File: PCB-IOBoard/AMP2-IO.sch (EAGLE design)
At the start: 85 parts, among them IC1 7404TS, IC2 R-78E6.5-0.5, IC3 REG1117, IC4 REG1117, K2 GN210S03, Q4 24.576, X3 MKDSN1,5/2-5,08

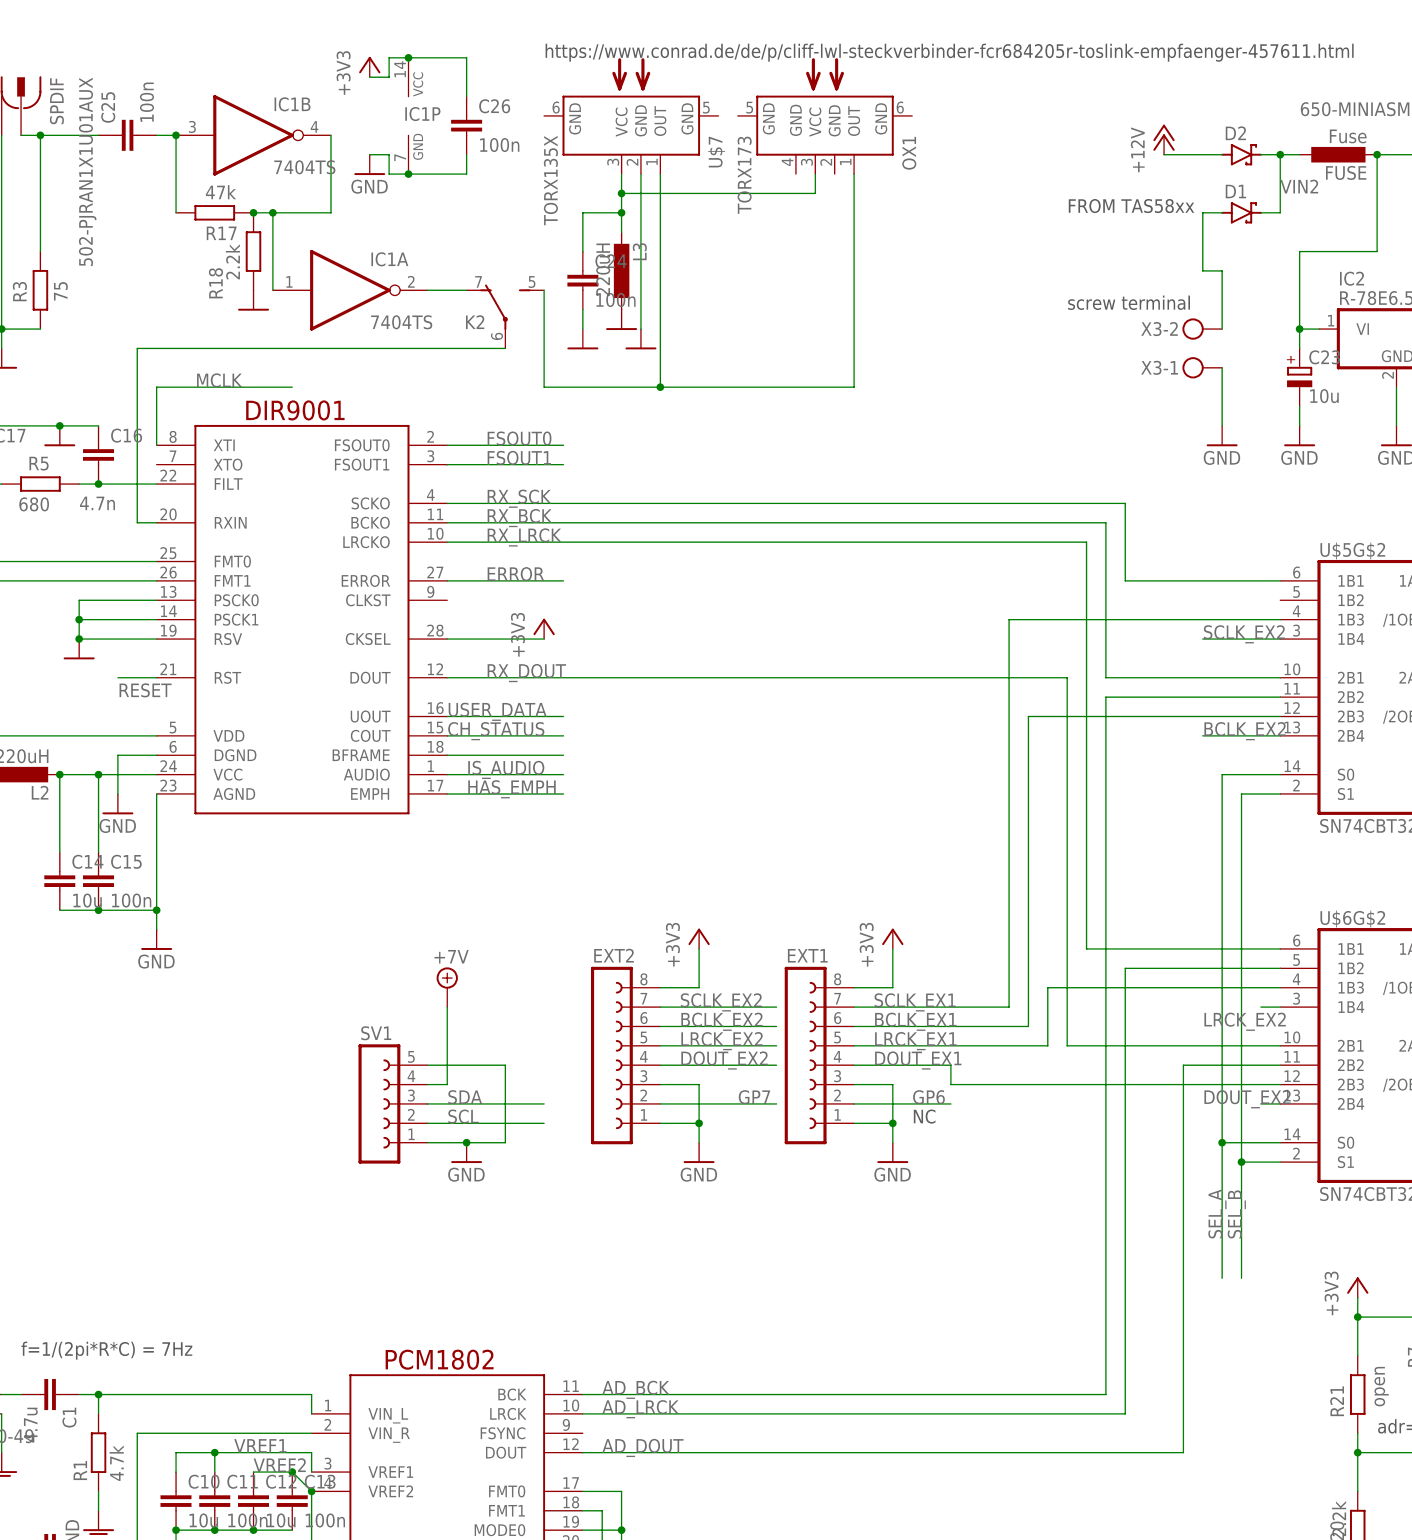
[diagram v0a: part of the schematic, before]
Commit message: Some RC1 bugs fixed.
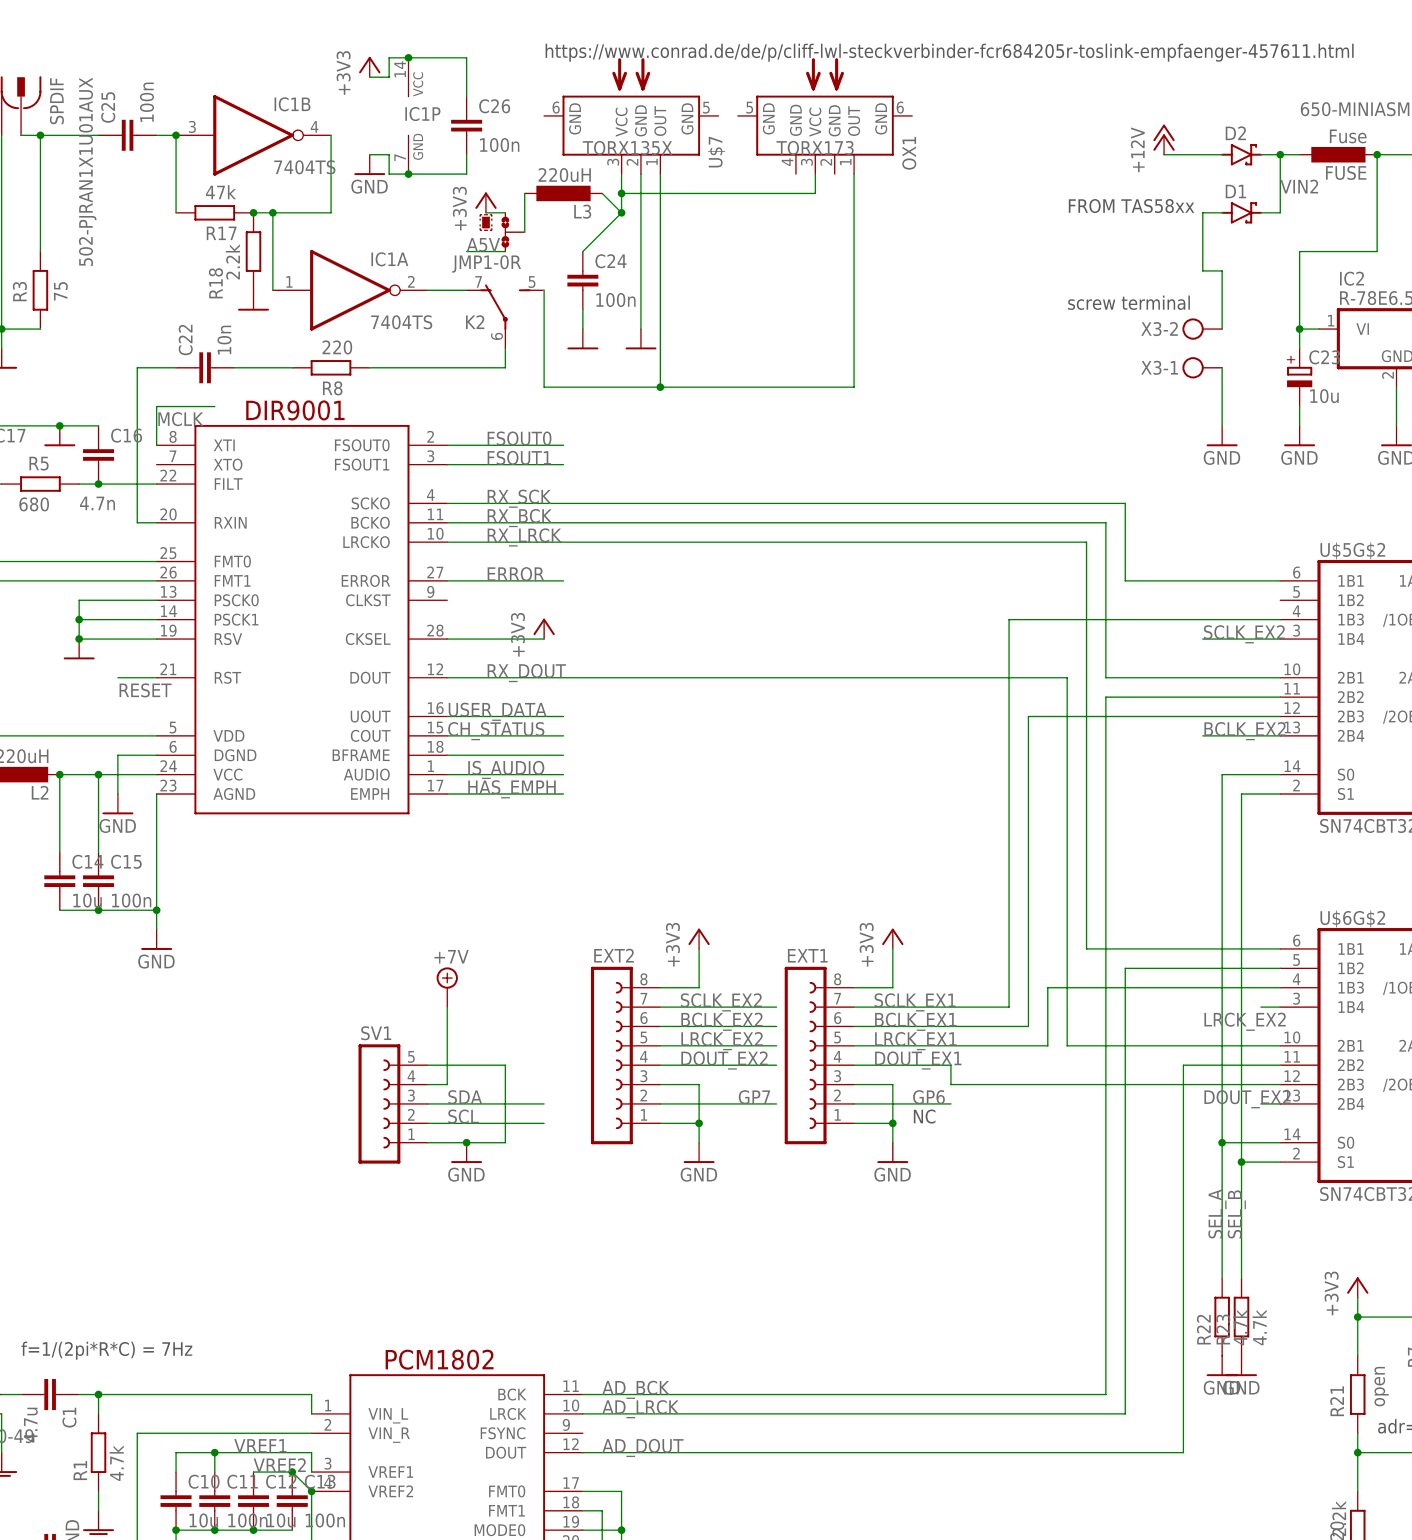
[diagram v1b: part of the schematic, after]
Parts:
- added C22: 10n, rcl:C-EUC0603
- added JMP1: 0R-JUMPA, jump-0r-smd:0R-JUMPA
- added R22, R23: 4.7k, rcl:R-EU_R0603
- added R8: 220, rcl:R-EU_R0603
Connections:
- new net N$6: JMP1-0R.2, L3.1
- new net N$7: C22.2, R8.1
- new net N$8: K2T.P, R8.2
- net +3V3: now also JMP1-0R.1
- net A5V: now also JMP1-0R.3
- net GND: now also R22.1, R23.1; no longer L3.1
- net N$19: now also C22.1; no longer K2T.P
- net SEL_A: now also R22.2
- net SEL_B: now also R23.2
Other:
- moved on the sheet: L3
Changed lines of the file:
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@@
 <part name="GND27" library="supply1" library_urn="urn:adsk.eagle:library:371" deviceset="GND" device=""/>
 <part name="GND28" library="supply1" library_urn="urn:adsk.eagle:library:371" deviceset="GND" device=""/>
-<part name="GND29" library="supply1" library_urn="urn:adsk.eagle:library:371" deviceset="GND" device=""/>
 <part name="GND30" library="supply1" library_urn="urn:adsk.eagle:library:371" deviceset="GND" device=""/>
 <part name="GND31" library="supply1" library_urn="urn:adsk.eagle:library:371" deviceset="GND" device=""/>
@@
 <part name="R7" library="rcl" library_urn="urn:adsk.eagle:library:334" deviceset="R-EU_" device="R0603" package3d_urn="urn:adsk.eagle:package:23555/3" value="2.2k"/>
 <part name="GND39" library="supply1" library_urn="urn:adsk.eagle:library:371" deviceset="GND" device=""/>
+<part name="JMP1" library="jump-0r-smd" library_urn="urn:adsk.eagle:library:251" deviceset="0R-JUMP" device="A" package3d_urn="urn:adsk.eagle:package:15385/1"/>
+<part name="+3V22" library="supply1" library_urn="urn:adsk.eagle:library:371" deviceset="+3V3" device=""/>
+<part name="C22" library="rcl" library_urn="urn:adsk.eagle:library:334" deviceset="C-EU" device="C0603" package3d_urn="urn:adsk.eagle:package:23616/2" value="10n"/>
+<part name="R8" library="rcl" library_urn="urn:adsk.eagle:library:334" deviceset="R-EU_" device="R0603" package3d_urn="urn:adsk.eagle:package:23555/3" value="220"/>
+<part name="R22" library="rcl" library_urn="urn:adsk.eagle:library:334" deviceset="R-EU_" device="R0603" package3d_urn="urn:adsk.eagle:package:23555/3" value="4.7k"/>
+<part name="R23" library="rcl" library_urn="urn:adsk.eagle:library:334" deviceset="R-EU_" device="R0603" package3d_urn="urn:adsk.eagle:package:23555/3" value="4.7k"/>
+<part name="GND29" library="supply1" library_urn="urn:adsk.eagle:library:371" deviceset="GND" device=""/>
+<part name="GND40" library="supply1" library_urn="urn:adsk.eagle:library:371" deviceset="GND" device=""/>
 </parts>
 <sheets>
@@
 <instance part="U$7" gate="G$1" x="96.52" y="248.92" smashed="yes" rot="R270">
 <attribute name="NAME" x="105.41" y="248.92" size="1.778" layer="95" rot="R270"/>
-<attribute name="VALUE" x="83.82" y="248.92" size="1.778" layer="96" rot="R270"/>
+<attribute name="VALUE" x="88.9" y="246.38" size="1.778" layer="96"/>
 <attribute name="MOUSER" x="96.52" y="248.92" size="1.778" layer="96" rot="R270" display="off"/>
 </instance>
-<instance part="L3" gate="G$1" x="93.98" y="231.14" smashed="yes" rot="R180">
-<attribute name="NAME" x="95.4786" y="234.95" size="1.778" layer="95" rot="R270"/>
-<attribute name="VALUE" x="90.678" y="234.95" size="1.778" layer="96" rot="R270"/>
-<attribute name="MOUSER" x="93.98" y="231.14" size="1.778" layer="96" rot="R180" display="off"/>
+<instance part="L3" gate="G$1" x="86.36" y="241.3" smashed="yes" rot="R90">
+<attribute name="NAME" x="90.17" y="239.8014" size="1.778" layer="95" rot="R180"/>
+<attribute name="VALUE" x="90.17" y="244.602" size="1.778" layer="96" rot="R180"/>
+<attribute name="MOUSER" x="86.36" y="241.3" size="1.778" layer="96" rot="R90" display="off"/>
 </instance>
 <instance part="C24" gate="G$1" x="88.9" y="231.14" smashed="yes">
@@
 </instance>
 <instance part="GND28" gate="1" x="96.52" y="220.98" smashed="yes"/>
-<instance part="GND29" gate="1" x="93.98" y="223.52" smashed="yes"/>
 <instance part="GND30" gate="1" x="88.9" y="220.98" smashed="yes"/>
 <instance part="GND31" gate="1" x="12.7" y="218.44" smashed="yes"/>
@@
 <instance part="OX1" gate="G$1" x="119.38" y="251.46" smashed="yes" rot="R270">
 <attribute name="NAME" x="130.81" y="248.92" size="1.778" layer="95" rot="R270"/>
-<attribute name="VALUE" x="109.22" y="248.92" size="1.778" layer="96" rot="R270"/>
+<attribute name="VALUE" x="114.3" y="246.38" size="1.778" layer="96"/>
 </instance>
 <instance part="U$5" gate="G$1" x="213.36" y="167.64" smashed="yes">
@@
 <instance part="GND39" gate="1" x="345.44" y="96.52" smashed="yes">
 <attribute name="VALUE" x="342.9" y="93.98" size="1.778" layer="96"/>
+</instance>
+<instance part="JMP1" gate="-0R" x="78.74" y="236.22" smashed="yes">
+<attribute name="NAME" x="71.882" y="231.394" size="1.778" layer="95"/>
+</instance>
+<instance part="JMP1" gate="G$2" x="76.2" y="238.76" smashed="yes"/>
+<instance part="+3V22" gate="G$1" x="76.2" y="241.3" smashed="yes">
+<attribute name="VALUE" x="73.66" y="236.22" size="1.778" layer="96" rot="R90"/>
+</instance>
+<instance part="C22" gate="G$1" x="38.1" y="218.44" smashed="yes" rot="R90">
+<attribute name="NAME" x="37.719" y="219.964" size="1.778" layer="95" rot="R90"/>
+<attribute name="VALUE" x="42.799" y="219.964" size="1.778" layer="96" rot="R90"/>
+</instance>
+<instance part="R8" gate="G$1" x="55.88" y="218.44" smashed="yes">
+<attribute name="NAME" x="54.61" y="214.8586" size="1.778" layer="95"/>
+<attribute name="VALUE" x="54.61" y="220.218" size="1.778" layer="96"/>
+</instance>
+<instance part="R22" gate="G$1" x="172.72" y="93.98" smashed="yes" rot="R90">
+<attribute name="NAME" x="171.2214" y="90.17" size="1.778" layer="95" rot="R90"/>
+<attribute name="VALUE" x="176.022" y="90.17" size="1.778" layer="96" rot="R90"/>
+</instance>
+<instance part="R23" gate="G$1" x="175.26" y="93.98" smashed="yes" rot="R90">
+<attribute name="NAME" x="173.7614" y="90.17" size="1.778" layer="95" rot="R90"/>
+<attribute name="VALUE" x="178.562" y="90.17" size="1.778" layer="96" rot="R90"/>
+</instance>
+<instance part="GND29" gate="1" x="172.72" y="86.36" smashed="yes">
+<attribute name="VALUE" x="170.18" y="83.82" size="1.778" layer="96"/>
+</instance>
+<instance part="GND40" gate="1" x="175.26" y="86.36" smashed="yes">
+<attribute name="VALUE" x="172.72" y="83.82" size="1.778" layer="96"/>
 </instance>
 </instances>
@@
 </segment>
 <segment>
-<pinref part="L3" gate="G$1" pin="1"/>
-<pinref part="GND29" gate="1" pin="GND"/>
-</segment>
-<segment>
 <pinref part="C24" gate="G$1" pin="2"/>
 <pinref part="GND30" gate="1" pin="GND"/>
@@
 <pinref part="GND39" gate="1" pin="GND"/>
 </segment>
+<segment>
+<pinref part="R22" gate="G$1" pin="1"/>
+<pinref part="GND29" gate="1" pin="GND"/>
+</segment>
+<segment>
+<pinref part="R23" gate="G$1" pin="1"/>
+<pinref part="GND40" gate="1" pin="GND"/>
+</segment>
 </net>
 <net name="A5V" class="0">
@@
 <junction x="58.42" y="35.56"/>
 <label x="48.26" y="35.56" size="1.778" layer="95"/>
+</segment>
+<segment>
+<pinref part="JMP1" gate="-0R" pin="3"/>
+<wire x1="78.74" y1="233.68" x2="73.66" y2="233.68" width="0.1524" layer="91"/>
+<label x="73.66" y="233.68" size="1.778" layer="95"/>
 </segment>
 </net>
@@
 <pinref part="+3V21" gate="G$1" pin="+3V3"/>
 </segment>
+<segment>
+<pinref part="JMP1" gate="-0R" pin="1"/>
+<pinref part="+3V22" gate="G$1" pin="+3V3"/>
+<wire x1="78.74" y1="238.76" x2="76.2" y2="238.76" width="0.1524" layer="91"/>
+</segment>
 </net>
 <net name="VREF1" class="0">
@@
 <pinref part="U$2" gate="G$1" pin="RXIN"/>
 <wire x1="33.02" y1="198.12" x2="30.48" y2="198.12" width="0.1524" layer="91"/>
-<wire x1="30.48" y1="198.12" x2="30.48" y2="220.98" width="0.1524" layer="91"/>
-<wire x1="78.74" y1="220.98" x2="30.48" y2="220.98" width="0.1524" layer="91"/>
-<pinref part="K2" gate="T" pin="P"/>
+<wire x1="30.48" y1="198.12" x2="30.48" y2="218.44" width="0.1524" layer="91"/>
+<wire x1="30.48" y1="218.44" x2="35.56" y2="218.44" width="0.1524" layer="91"/>
+<pinref part="C22" gate="G$1" pin="1"/>
 </segment>
 </net>
@@
 <pinref part="U$5" gate="G$2" pin="S1"/>
 <pinref part="U$6" gate="G$2" pin="S1"/>
+<pinref part="R23" gate="G$1" pin="2"/>
 </segment>
 <segment>
@@
 <pinref part="U$5" gate="G$2" pin="S0"/>
 <pinref part="U$6" gate="G$2" pin="S0"/>
+<pinref part="R22" gate="G$1" pin="2"/>
 </segment>
 <segment>
@@
 <segment>
 <pinref part="U$2" gate="G$1" pin="XTI"/>
-<wire x1="33.02" y1="208.28" x2="33.02" y2="215.9" width="0.1524" layer="91"/>
-<wire x1="33.02" y1="215.9" x2="50.8" y2="215.9" width="0.1524" layer="91"/>
-<label x="38.1" y="215.9" size="1.778" layer="95"/>
+<wire x1="33.02" y1="208.28" x2="33.02" y2="213.36" width="0.1524" layer="91"/>
+<wire x1="33.02" y1="213.36" x2="40.64" y2="213.36" width="0.1524" layer="91"/>
+<label x="33.02" y="210.82" size="1.778" layer="95"/>
 </segment>
 </net>
@@
 <pinref part="L3" gate="G$1" pin="2"/>
 <pinref part="U$7" gate="G$1" pin="VCC"/>
-<wire x1="93.98" y1="236.22" x2="93.98" y2="238.76" width="0.1524" layer="91"/>
+<wire x1="91.44" y1="241.3" x2="93.98" y2="238.76" width="0.1524" layer="91"/>
 <pinref part="C24" gate="G$1" pin="1"/>
 <wire x1="93.98" y1="238.76" x2="93.98" y2="241.3" width="0.1524" layer="91"/>
 <wire x1="93.98" y1="241.3" x2="93.98" y2="243.84" width="0.1524" layer="91"/>
-<wire x1="88.9" y1="233.68" x2="88.9" y2="238.76" width="0.1524" layer="91"/>
-<wire x1="88.9" y1="238.76" x2="93.98" y2="238.76" width="0.1524" layer="91"/>
+<wire x1="88.9" y1="233.68" x2="93.98" y2="238.76" width="0.1524" layer="91"/>
 <junction x="93.98" y="238.76"/>
 <pinref part="OX1" gate="G$1" pin="VCC"/>
@@
 </segment>
 </net>
+<net name="N$6" class="0">
+<segment>
+<pinref part="L3" gate="G$1" pin="1"/>
+<pinref part="JMP1" gate="-0R" pin="2"/>
+<wire x1="81.28" y1="241.3" x2="81.28" y2="236.22" width="0.1524" layer="91"/>
+</segment>
+</net>
+<net name="N$7" class="0">
+<segment>
+<pinref part="C22" gate="G$1" pin="2"/>
+<pinref part="R8" gate="G$1" pin="1"/>
+<wire x1="43.18" y1="218.44" x2="50.8" y2="218.44" width="0.1524" layer="91"/>
+</segment>
+</net>
+<net name="N$8" class="0">
+<segment>
+<pinref part="R8" gate="G$1" pin="2"/>
+<pinref part="K2" gate="T" pin="P"/>
+<wire x1="60.96" y1="218.44" x2="78.74" y2="218.44" width="0.1524" layer="91"/>
+<wire x1="78.74" y1="218.44" x2="78.74" y2="220.98" width="0.1524" layer="91"/>
+</segment>
+</net>
